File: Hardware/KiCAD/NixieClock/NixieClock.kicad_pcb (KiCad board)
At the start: 2 copper layers, 6 parts, among them IC1 , IC2 

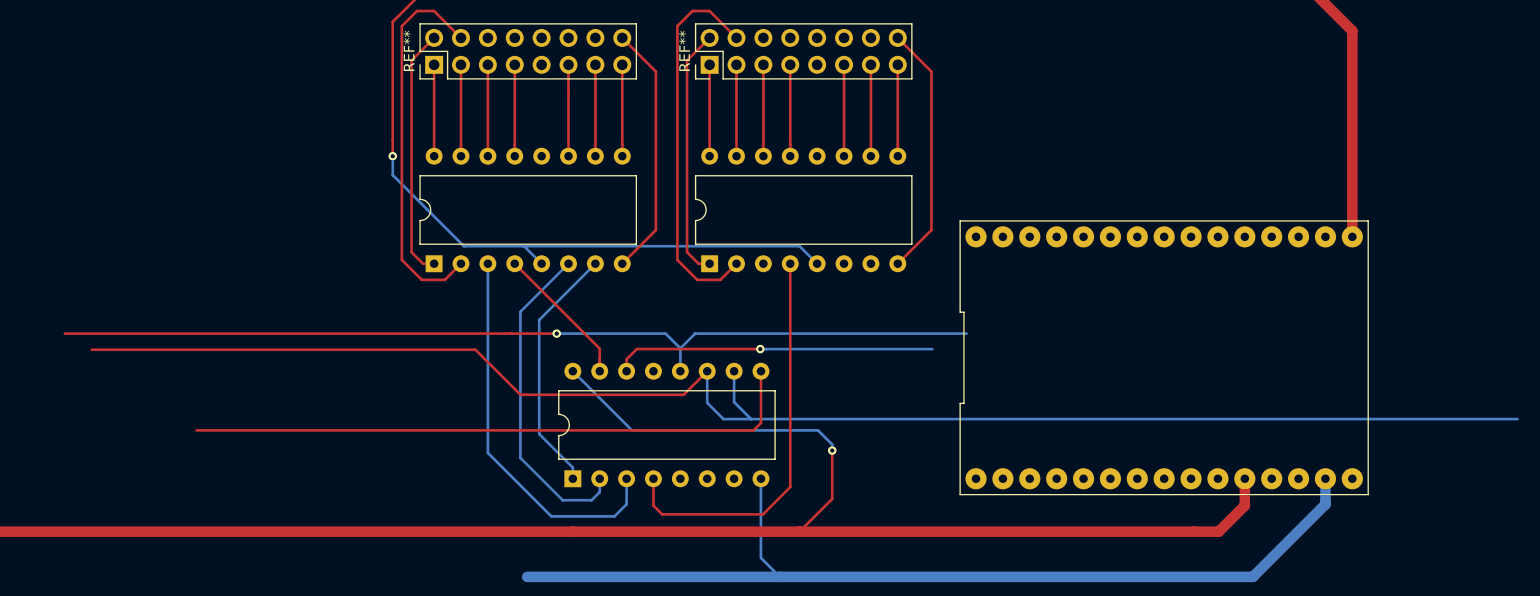
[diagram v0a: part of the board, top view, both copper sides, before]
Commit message: Progress.. about to duplicate to 3 stages
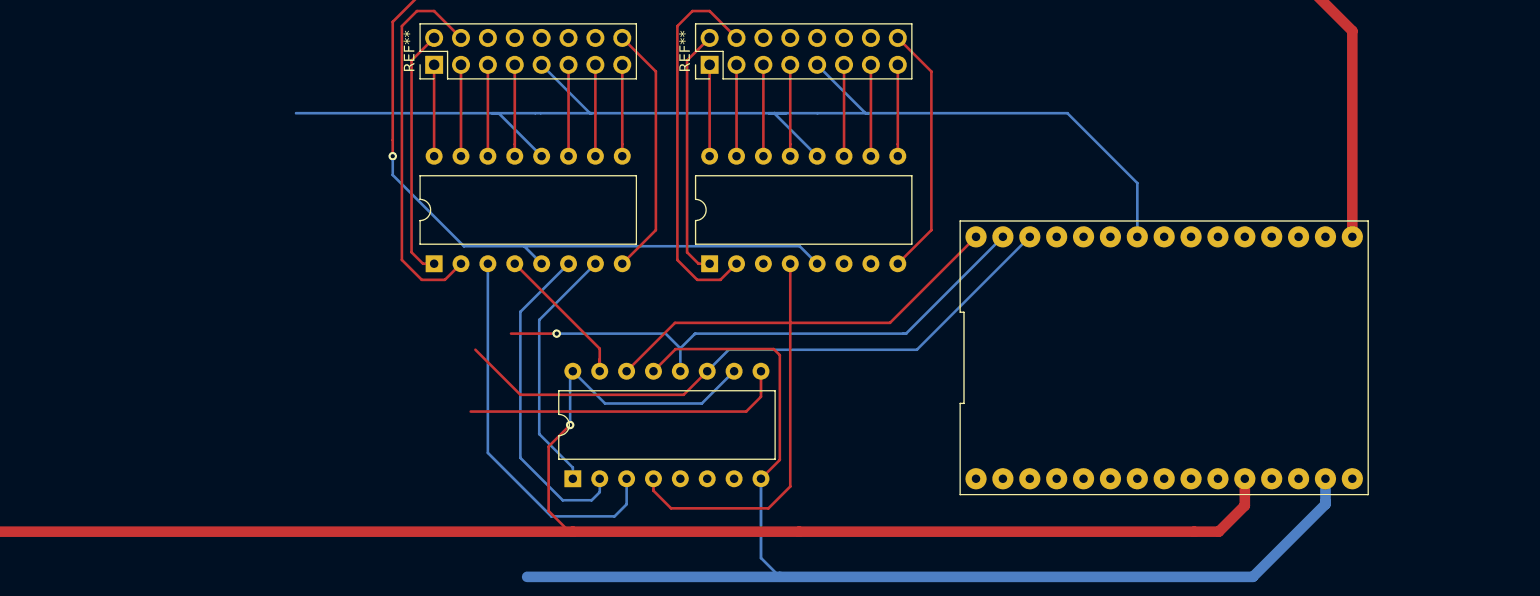
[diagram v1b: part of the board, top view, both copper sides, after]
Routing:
- net (no net): track 1473.9 -> 1469.5 mm, vias 4 -> 3
